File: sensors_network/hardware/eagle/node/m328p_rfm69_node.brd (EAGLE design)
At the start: 65.5 x 39.9 mm, 32 parts, among them IC2 L6920, U1 M328P, U2 RFM69W, Y1 8MHz

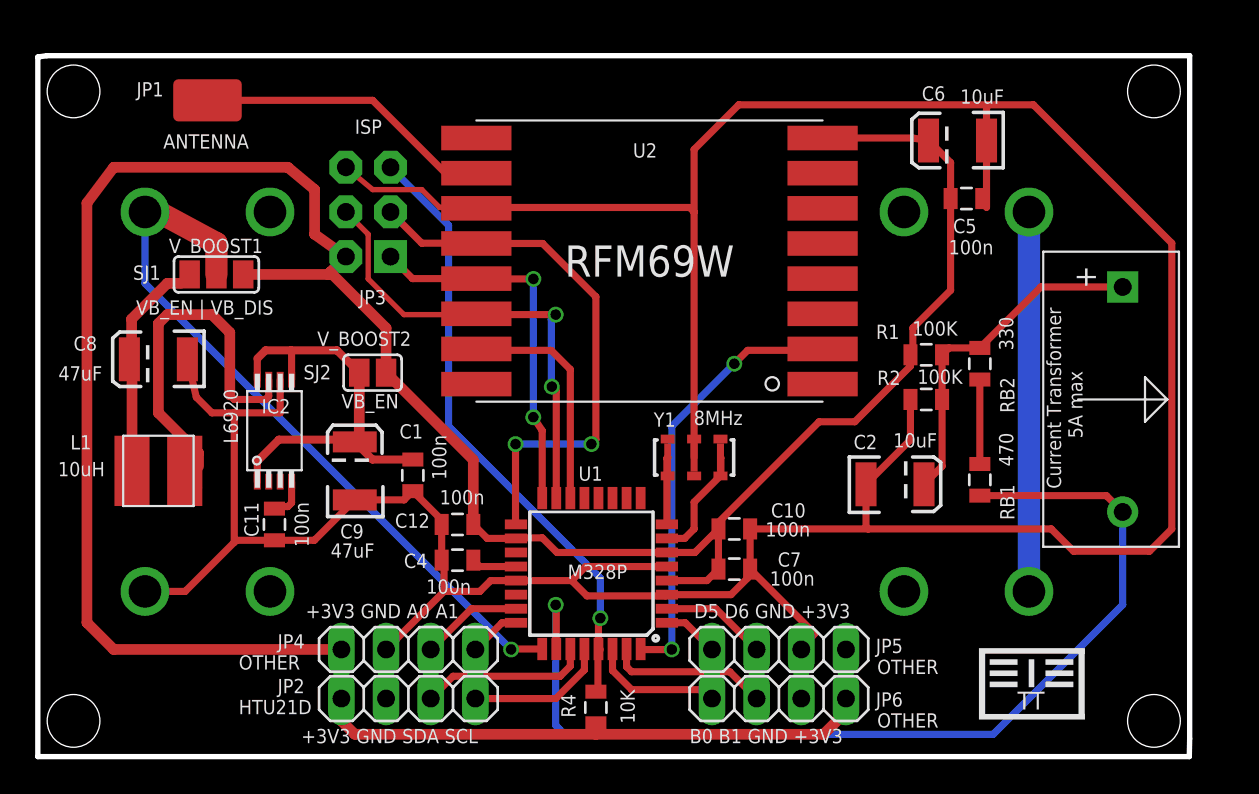
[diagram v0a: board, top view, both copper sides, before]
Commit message: [sensors network] small pcb/schematic final touches
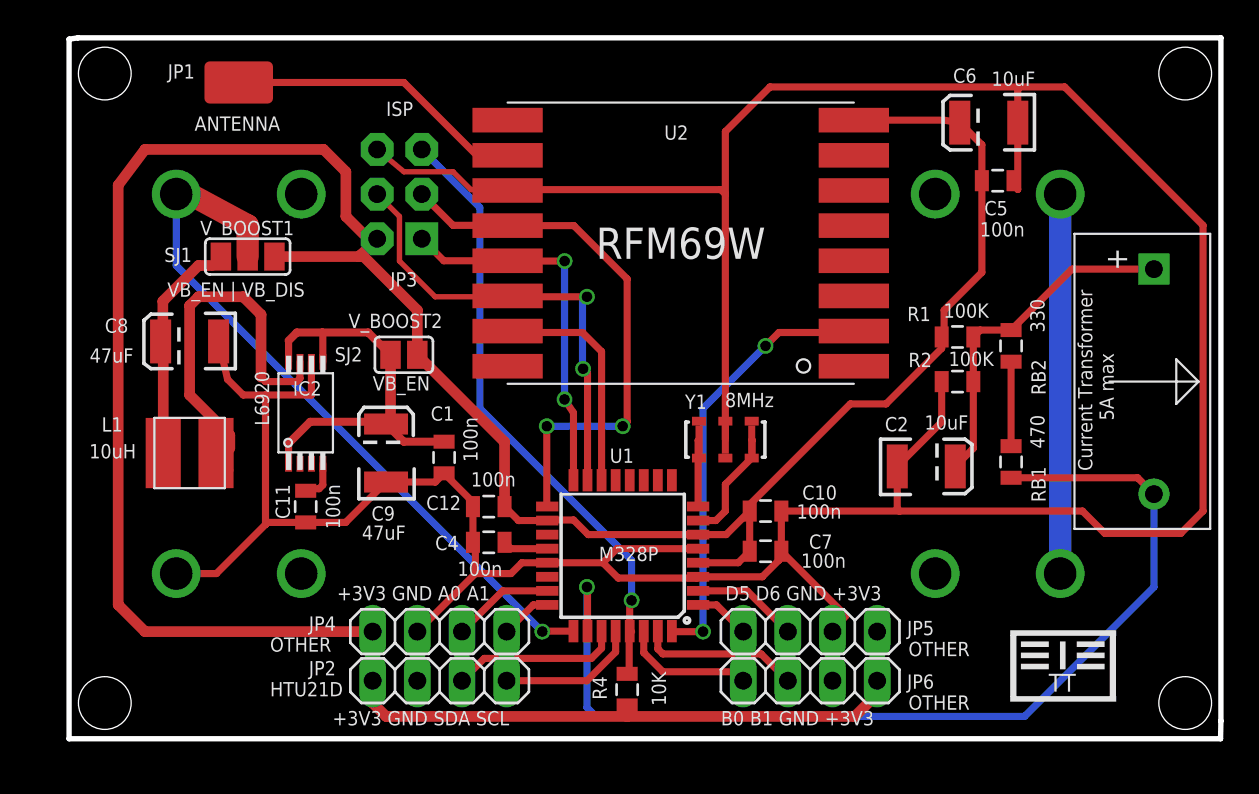
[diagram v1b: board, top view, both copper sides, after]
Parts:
- moved C6 2.05 mm to (52.6, 35.1)
- moved C8 2.05 mm to (7.11, 22.6)
- moved JP3 2.05 mm to (19.1, 31.0)
- moved L1 2.05 mm to (7.11, 16.3)
- moved CT1 2.05 mm to (62.0, 20.3)
- moved IC2 2.05 mm to (13.7, 18.5)
- moved R2 2.05 mm to (50.8, 20.3)
- moved RB2 2.05 mm to (53.8, 22.4)
- moved SJ2 2.05 mm to (19.3, 21.8)
- moved Y1 2.05 mm to (37.6, 17.0)
- moved JP1 2.05 mm to (9.91, 37.3)
- moved SJ1 2.05 mm to (10.4, 27.4)
- moved BAT4 2.05 mm to (31.5, 9.40)
- moved C10 2.05 mm to (39.9, 13.0)
- moved C11 2.05 mm to (13.7, 13.2)
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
